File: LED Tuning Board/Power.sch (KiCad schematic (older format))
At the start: 13 parts, among them J1 Jack-DC, J2 V_SEL, J3 V_ADJ, U1 LM317_TO-220

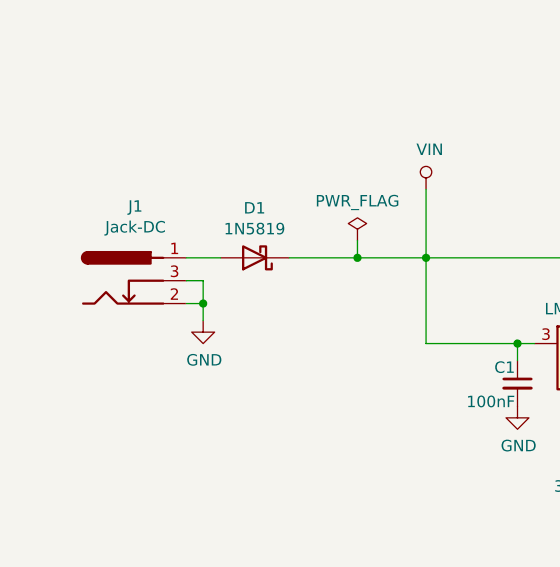
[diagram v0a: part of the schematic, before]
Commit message: Added layout
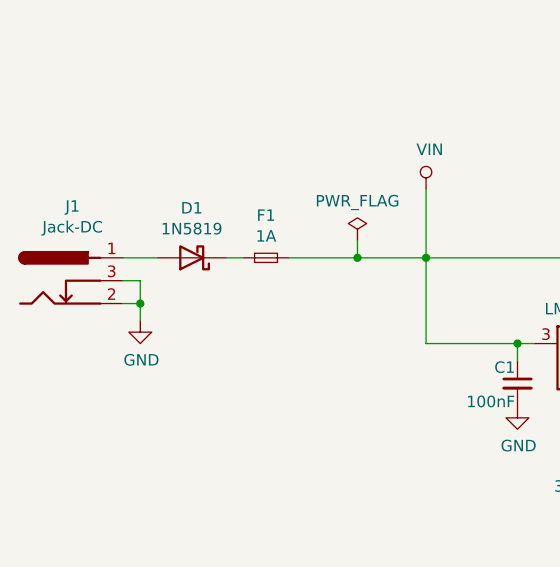
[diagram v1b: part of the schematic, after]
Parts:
- added F1: 1A, fuse_holder:Fuseholder5x20_horiz_SemiClosed_Casing10x25mm, symbol Device:Fuse_Small
- C2: footprint (none) -> Capacitor_THT:CP_Radial_D4.0mm_P2.00mm
- J1: footprint (none) -> power:BARREL_JACK
- J2: footprint (none) -> Connector_PinHeader_2.54mm:PinHeader_2x02_P2.54mm_Vertical
- J3: footprint (none) -> Connector_PinHeader_2.54mm:PinHeader_2x03_P2.54mm_Vertical
- R1, R2, R3, R4: footprint (none) -> resistor:R_Axial_DIN0207_L6.3mm_D2.5mm_P10.16mm_Horizontal
- TP1, TP2: footprint (none) -> testpoint:TestPoint
- U1: footprint Package_TO_SOT_THT:TO-220-3_Vertical -> Package_TO_SOT_THT:TO-220-3_Horizontal_TabDown
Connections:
- net VIN: now also F1.2; no longer D1.1 (K)
- new net: D1.1 (K), F1.1
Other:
- moved on the sheet: D1, J1
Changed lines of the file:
@@
 F 0 "U1" H 5950 3342 50  0000 C CNN
 F 1 "LM317_TO-220" H 5950 3251 50  0000 C CNN
-F 2 "Package_TO_SOT_THT:TO-220-3_Vertical" H 5950 3350 50  0001 C CIN
+F 2 "Package_TO_SOT_THT:TO-220-3_Horizontal_TabDown" H 5950 3350 50  0001 C CIN
 F 3 "http://www.ti.com/lit/ds/symlink/lm317.pdf" H 5950 3100 50  0001 C CNN
 	1    5950 3100
@@
 F 0 "R1" H 6395 3371 50  0000 L CNN
 F 1 "240*" H 6395 3280 50  0000 L CNN
-F 2 "" V 6255 3325 50  0001 C CNN
+F 2 "resistor:R_Axial_DIN0207_L6.3mm_D2.5mm_P10.16mm_Horizontal" V 6255 3325 50  0001 C CNN
 F 3 "~" H 6325 3325 50  0001 C CNN
 	1    6325 3325
@@
 F 0 "C2" H 6763 3321 50  0000 L CNN
 F 1 "1uF" H 6763 3230 50  0000 L CNN
-F 2 "" H 6675 3275 50  0001 C CNN
+F 2 "Capacitor_THT:CP_Radial_D4.0mm_P2.00mm" H 6675 3275 50  0001 C CNN
 F 3 "~" H 6675 3275 50  0001 C CNN
 	1    6675 3275
@@
 L barrel_jack:Jack-DC J?
 U 1 1 6440E550
-P 3825 2825
+P 3550 2825
 AR Path="/6440E550" Ref="J?"  Part="1"
 AR Path="/643F8439/6440E550" Ref="J1"  Part="1"
-F 0 "J1" H 3904 3150 50  0000 C CNN
-F 1 "Jack-DC" H 3904 3059 50  0000 C CNN
-F 2 "" H 3875 2785 50  0001 C CNN
-F 3 "~" H 3875 2785 50  0001 C CNN
-	1    3825 2825
+F 0 "J1" H 3629 3150 50  0000 C CNN
+F 1 "Jack-DC" H 3629 3059 50  0000 C CNN
+F 2 "power:BARREL_JACK" H 3600 2785 50  0001 C CNN
+F 3 "~" H 3600 2785 50  0001 C CNN
+	1    3550 2825
 	1    0    0    -1
 $EndComp
@@
 $EndComp
 Wire Wire Line
-	4125 2825 4200 2825
-Wire Wire Line
-	4200 2825 4200 2925
-Wire Wire Line
-	4200 2925 4125 2925
-Wire Wire Line
-	4200 2925 4200 3000
-Connection ~ 4200 2925
+	3850 2825 3925 2825
+Wire Wire Line
+	3925 2825 3925 2925
+Wire Wire Line
+	3925 2925 3850 2925
+Wire Wire Line
+	3925 2925 3925 3000
+Connection ~ 3925 2925
 $Comp
 L power:GND #PWR?
 U 1 1 6440E561
-P 4200 3000
+P 3925 3000
 AR Path="/6440E561" Ref="#PWR?"  Part="1"
 AR Path="/643F8439/6440E561" Ref="#PWR01"  Part="1"
-F 0 "#PWR01" H 4200 2750 50  0001 C CNN
-F 1 "GND" H 4205 2827 50  0000 C CNN
-F 2 "" H 4200 3000 50  0001 C CNN
-F 3 "" H 4200 3000 50  0001 C CNN
-	1    4200 3000
+F 0 "#PWR01" H 3925 2750 50  0001 C CNN
+F 1 "GND" H 3930 2827 50  0000 C CNN
+F 2 "" H 3925 3000 50  0001 C CNN
+F 3 "" H 3925 3000 50  0001 C CNN
+	1    3925 3000
 	1    0    0    -1
 $EndComp
@@
 F 0 "R2" H 5975 3950 50  0000 L CNN
 F 1 "390*" H 6000 3875 50  0000 L CNN
-F 2 "" V 5880 3800 50  0001 C CNN
+F 2 "resistor:R_Axial_DIN0207_L6.3mm_D2.5mm_P10.16mm_Horizontal" V 5880 3800 50  0001 C CNN
 F 3 "~" H 5950 3800 50  0001 C CNN
 	1    5950 3800
@@
 F 0 "J3" V 6154 4112 50  0000 R CNN
 F 1 "V_ADJ" V 6245 4112 50  0000 R CNN
-F 2 "" H 6150 4300 50  0001 C CNN
+F 2 "Connector_PinHeader_2.54mm:PinHeader_2x03_P2.54mm_Vertical" H 6150 4300 50  0001 C CNN
 F 3 "~" H 6150 4300 50  0001 C CNN
 	1    6150 4300
@@
 F 0 "R3" H 6175 3950 50  0000 L CNN
 F 1 "*" H 6200 3875 50  0000 L CNN
-F 2 "" V 6080 3800 50  0001 C CNN
+F 2 "resistor:R_Axial_DIN0207_L6.3mm_D2.5mm_P10.16mm_Horizontal" V 6080 3800 50  0001 C CNN
 F 3 "~" H 6150 3800 50  0001 C CNN
 	1    6150 3800
@@
 F 0 "R4" H 6325 3950 50  0000 L CNN
 F 1 "*" H 6375 3875 50  0000 L CNN
-F 2 "" V 6255 3800 50  0001 C CNN
+F 2 "resistor:R_Axial_DIN0207_L6.3mm_D2.5mm_P10.16mm_Horizontal" V 6255 3800 50  0001 C CNN
 F 3 "~" H 6325 3800 50  0001 C CNN
 	1    6325 3800
@@
 F 0 "J2" H 7525 2942 50  0000 C CNN
 F 1 "V_SEL" H 7525 2851 50  0000 C CNN
-F 2 "" H 7475 2725 50  0001 C CNN
+F 2 "Connector_PinHeader_2.54mm:PinHeader_2x02_P2.54mm_Vertical" H 7475 2725 50  0001 C CNN
 F 3 "~" H 7475 2725 50  0001 C CNN
 	1    7475 2725
@@
 L Diode:1N5819 D?
 U 1 1 6440E5AB
-P 4425 2725
+P 4150 2725
 AR Path="/6440E5AB" Ref="D?"  Part="1"
 AR Path="/643F8439/6440E5AB" Ref="D1"  Part="1"
-F 0 "D1" H 4425 2508 50  0000 C CNN
-F 1 "1N5819" H 4425 2599 50  0000 C CNN
-F 2 "Diode_THT:D_DO-41_SOD81_P10.16mm_Horizontal" H 4425 2550 50  0001 C CNN
-F 3 "http://www.vishay.com/docs/88525/1n5817.pdf" H 4425 2725 50  0001 C CNN
-	1    4425 2725
+F 0 "D1" H 4150 2508 50  0000 C CNN
+F 1 "1N5819" H 4150 2599 50  0000 C CNN
+F 2 "Diode_THT:D_DO-41_SOD81_P10.16mm_Horizontal" H 4150 2550 50  0001 C CNN
+F 3 "http://www.vishay.com/docs/88525/1n5817.pdf" H 4150 2725 50  0001 C CNN
+	1    4150 2725
 	-1   0    0    1
 $EndComp
 Wire Wire Line
-	4125 2725 4275 2725
+	3850 2725 4000 2725
 $Comp
 L power:PWR_FLAG #FLG?
@@
 F 0 "TP1" V 7954 3013 50  0000 L CNN
 F 1 "TP_VCC" V 8045 3013 50  0000 L CNN
-F 2 "" H 8200 2825 50  0001 C CNN
+F 2 "testpoint:TestPoint" H 8200 2825 50  0001 C CNN
 F 3 "~" H 8200 2825 50  0001 C CNN
 	1    8000 2825
@@
 F 0 "TP2" V 7954 3213 50  0000 L CNN
 F 1 "TP_GND" V 8045 3213 50  0000 L CNN
-F 2 "" H 8200 3025 50  0001 C CNN
+F 2 "testpoint:TestPoint" H 8200 3025 50  0001 C CNN
 F 3 "~" H 8200 3025 50  0001 C CNN
 	1    8000 3025
@@
 Wire Wire Line
 	7850 3025 7850 3125
+$Comp
+L Device:Fuse_Small F1
+U 1 1 643D5E84
+P 4475 2725
+F 0 "F1" H 4475 2910 50  0000 C CNN
+F 1 "1A" H 4475 2819 50  0000 C CNN
+F 2 "fuse_holder:Fuseholder5x20_horiz_SemiClosed_Casing10x25mm" H 4475 2725 50  0001 C CNN
+F 3 "~" H 4475 2725 50  0001 C CNN
+	1    4475 2725
+	1    0    0    -1
+$EndComp
+Wire Wire Line
+	4300 2725 4375 2725
 $EndSCHEMATC
